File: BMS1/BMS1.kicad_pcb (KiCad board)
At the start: 2 copper layers, 313 x 155.7 mm, 210 parts, among them J1 Conn_01x02, J2 Conn_01x02, J3 Conn_01x02, Q1 Q_NPN_BCE, Q2 DXT5551P5-13_DIO, T1 ESMIT-4180_C, U1 ADG728, U10 LTC6812-1, U2 ADG728, U3 ADG728, U4 ADG728, U5 ADG728, U6 ADG728, U7 ADG728, U8 ADG728, U9 LTC6812-1

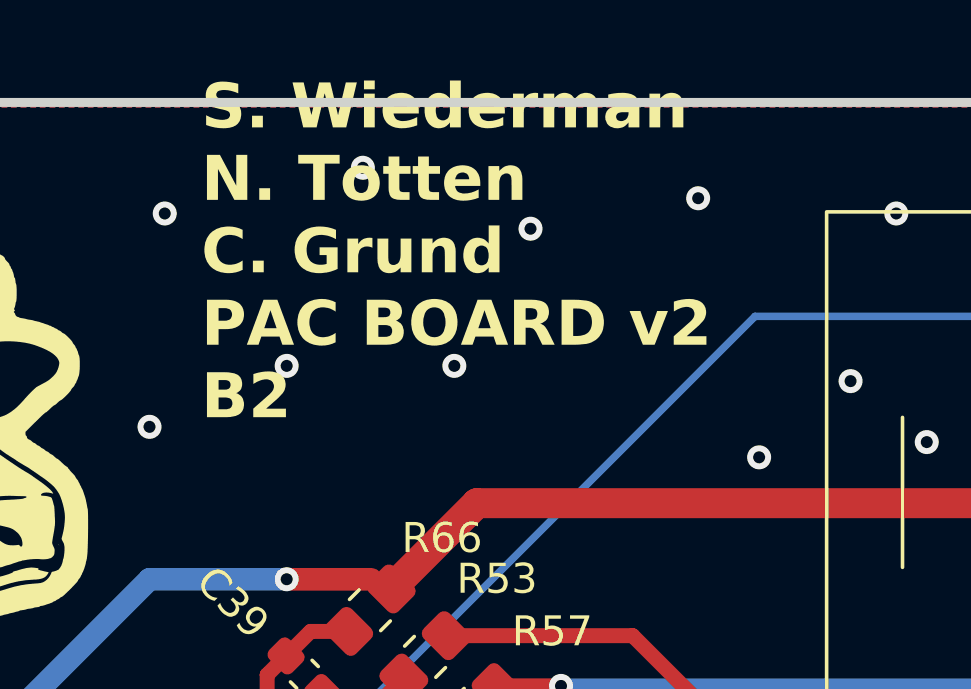
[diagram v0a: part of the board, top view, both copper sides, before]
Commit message: Footprints
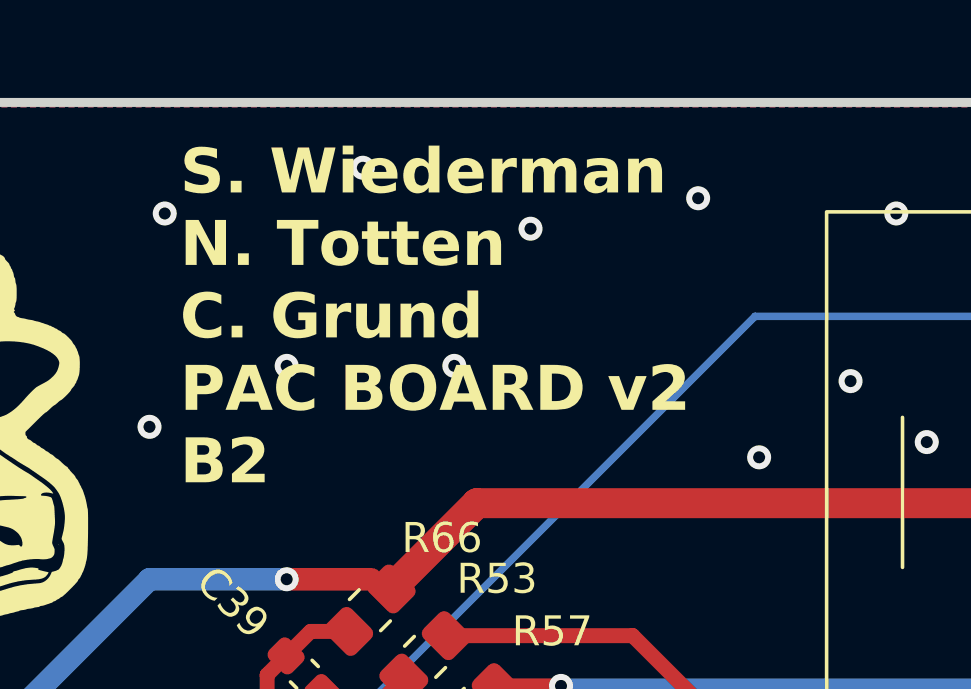
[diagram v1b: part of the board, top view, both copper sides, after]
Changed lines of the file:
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@@
 		(tags "capacitor handsolder")
 		(property "Reference" "C42"
-			(at 0 -1.43 360)
+			(at 0 -1.43 0)
 			(layer "F.SilkS")
 			(effects
@@
 		)
 		(property "Value" "1uf"
-			(at 0 1.43 360)
+			(at 0 1.43 0)
 			(layer "F.Fab")
 			(effects
@@
 		)
 		(fp_text user "${REFERENCE}"
-			(at -1.6775 1.27 360)
+			(at -1.6775 1.27 0)
 			(layer "F.Fab")
 			(effects
@@
 	)
 	(gr_text "S. Wiederman\nN. Totten\nC. Grund\nPAC BOARD v2\nB2"
-		(at 54.05 30.85 0)
+		(at 53.34 33.02 0)
 		(layer "F.SilkS")
 		(effects
